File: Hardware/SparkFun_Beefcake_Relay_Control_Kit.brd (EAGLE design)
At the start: 58.4 x 27.9 mm, 17 parts, among them Q2 2N3904, U6 RELAYPTH3

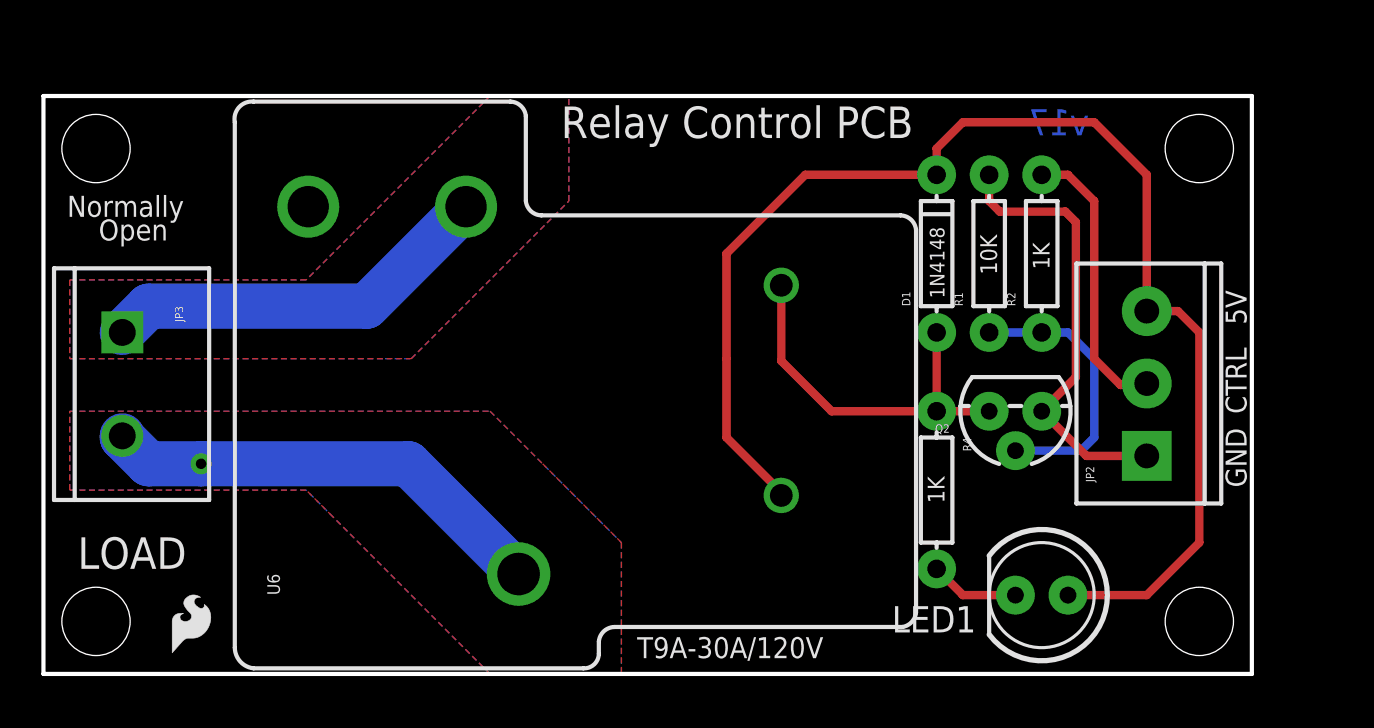
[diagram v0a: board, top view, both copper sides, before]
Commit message: Design ready for proto 1 review
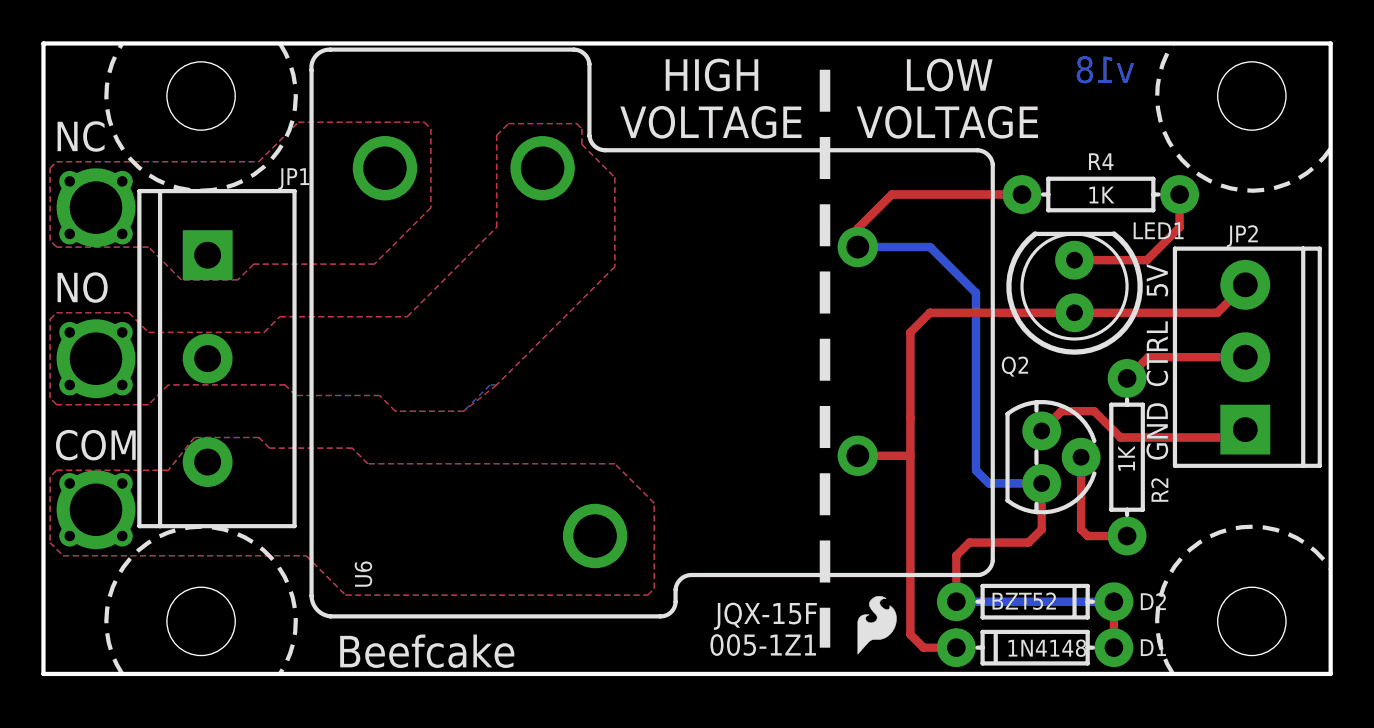
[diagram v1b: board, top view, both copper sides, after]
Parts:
- removed FRAME1: FRAME-LETTER, SparkFun-Aesthetics:CREATIVE_COMMONS
- removed JP3: Load, SparkFun:SCREWTERMINAL-5MM-2
- removed R1: 10K, SparkFun:AXIAL-0.3
- removed U$1: LOGO-SFENEW, SparkFun:SFE-NEW-WEBLOGO
- added D2: BZT52, SparkFun-DiscreteSemi:DIODE-BZT52
- added FRAME2: FRAME-LETTER, SparkFun-Aesthetics:CREATIVE_COMMONS
- added JP1: (no value), SparkFun-Connectors:SCREWTERMINAL-5MM-3
- added LOGO1: SFE_LOGO_NAME_FLAME.2_INCH, SparkFun-Aesthetics:SFE_LOGO_NAME_FLAME_.2
- D1: device SparkFun:DIODE-1N4148 -> SparkFun-DiscreteSemi:DIODE-1N4148
- JP2: device SparkFun:SCREWTERMINAL-3.5MM-3 -> SparkFun-Connectors:SCREWTERMINAL-3.5MM-3
- LED1: device SparkFun:LED5MM -> SparkFun-LED:LED5MM
- Q2: device SparkFun:TO-92 -> SparkFun-DiscreteSemi:TO-92
- R2, R4: device SparkFun:AXIAL-0.3 -> SparkFun-Resistors:AXIAL-0.3
- U6: value RELAYPTH3 -> JQX-15F; device SparkFun:RELAY-T9A-2 -> SparkFun-Electromechanical:RELAY-T90
- moved U$11 33.1 mm to (39.4, 0.95)
- moved U$12 27.2 mm to (51.8, 26.7)
- moved D1 19.6 mm to (47.9, 1.27), turned to 180 degrees
- moved U6 16.7 mm to (39.4, 24.4), turned to 0 degrees
- moved R4 16.3 mm to (51.1, 23.2), turned to 0 degrees
- moved LED1 15.0 mm to (49.8, 18.7), turned to 90 degrees
- moved R2 10.7 mm to (52.4, 10.5)
- moved U$7 5.68 mm to (7.62, 27.9)
- moved U$3 5.08 mm to (7.62, 2.54)
- moved JP2 4.93 mm to (58.1, 11.8)
- moved U$5 3.59 mm to (58.4, 27.9)
- moved Q2 2.56 mm to (48.3, 10.5), turned to 270 degrees
- moved U$4 2.54 mm to (58.4, 2.54)
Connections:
- removed net LOAD1: JP3.2, U6.MAIN
- removed net LOAD2: JP3.1, U6.NO
- new net COMMON: JP1.3, U6.MAIN
- new net NC: JP1.1, U6.NC
- new net NO: JP1.2, U6.NO
- net COIL: now also D2.A, D2.C
- net GND: no longer R1.P$2
- net N$6: no longer R1.P$1
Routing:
- net COIL: track 18.5 -> 47.1 mm
- net RAW: track 64.7 -> 36.8 mm
- net LOAD1: track 22.0 -> 0.00 mm, vias 1 -> 0
- net LOAD2: track 19.1 -> 0.00 mm
- net GND: track 21.7 -> 10.9 mm
- net RELAY: track 13.8 -> 6.14 mm
- net N$6: track 13.5 -> 5.85 mm
- net N$9: track 4.34 -> 7.33 mm
- added copper zone on layer 1, net COMMON
- added copper zone on layer 16, net COMMON
- added copper zone on layer 1, net NC
- added copper zone on layer 16, net NC
- added copper zone on layer 1, net NO
- added copper zone on layer 16, net NO
- removed copper zone on layer 1, net LOAD1
- removed copper zone on layer 16, net LOAD1
- removed copper zone on layer 1, net LOAD2
- removed copper zone on layer 16, net LOAD2
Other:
- board size 58.4 x 27.9 mm -> 62.2 x 30.5 mm
- board text added: "Beefcake"
- board text added: "Beefcake Relay Control"
- board text added: "COM"
- board text added: "CUT FOR ZENER USE"
- board text added: "HIGH VOLTAGE"
- board text added: "JQX-15F 005-1Z1"
- board text added: "LOW VOLTAGE"
- board text added: "NC"
- board text added: "NO"
- board text added: "Units in inches"
- board text added: "v18"
- board text removed: "LOAD"
- board text removed: "Normally"
- board text removed: "Open"
- board text removed: "Relay Control PCB"
- board text removed: "T9A-30A/120V"
- board text removed: "v17"
